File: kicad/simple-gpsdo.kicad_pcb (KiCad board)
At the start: 2 copper layers, 119.5 x 74.5 mm, 103 parts, among them J1 PPS_OUT, J2 PWR, J3 ISP, J4 GPS_NEO, J5 GPS_IN, J6 10MHz_OUT, J7 NEO-6M, J8 10MHz_OUT, J9 USB_C, Q1 DMP3099L, SW1 RST, U1 BD50FC0FP-E2, U2 ATmega32U4-AU, U3 MC74HC390, U4 CD74HC4046AM96, U5 BD50FC0FP-E2, U6 LM7171, U7 LM7171, U8 LM35-D, U9 AP62301WU-7, Y1 16MHz, Y2 NV47X

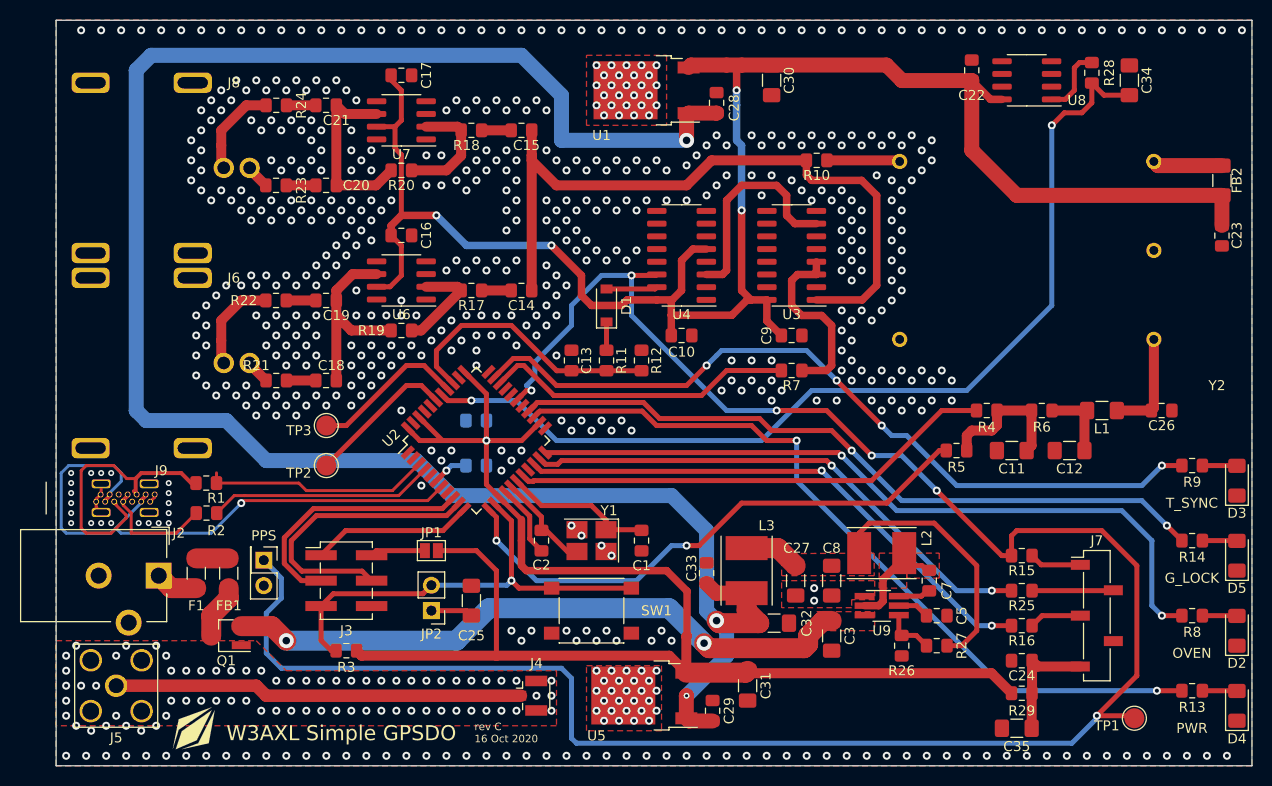
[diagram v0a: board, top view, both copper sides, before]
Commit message: schematic cleanup and re-plot of gerber files
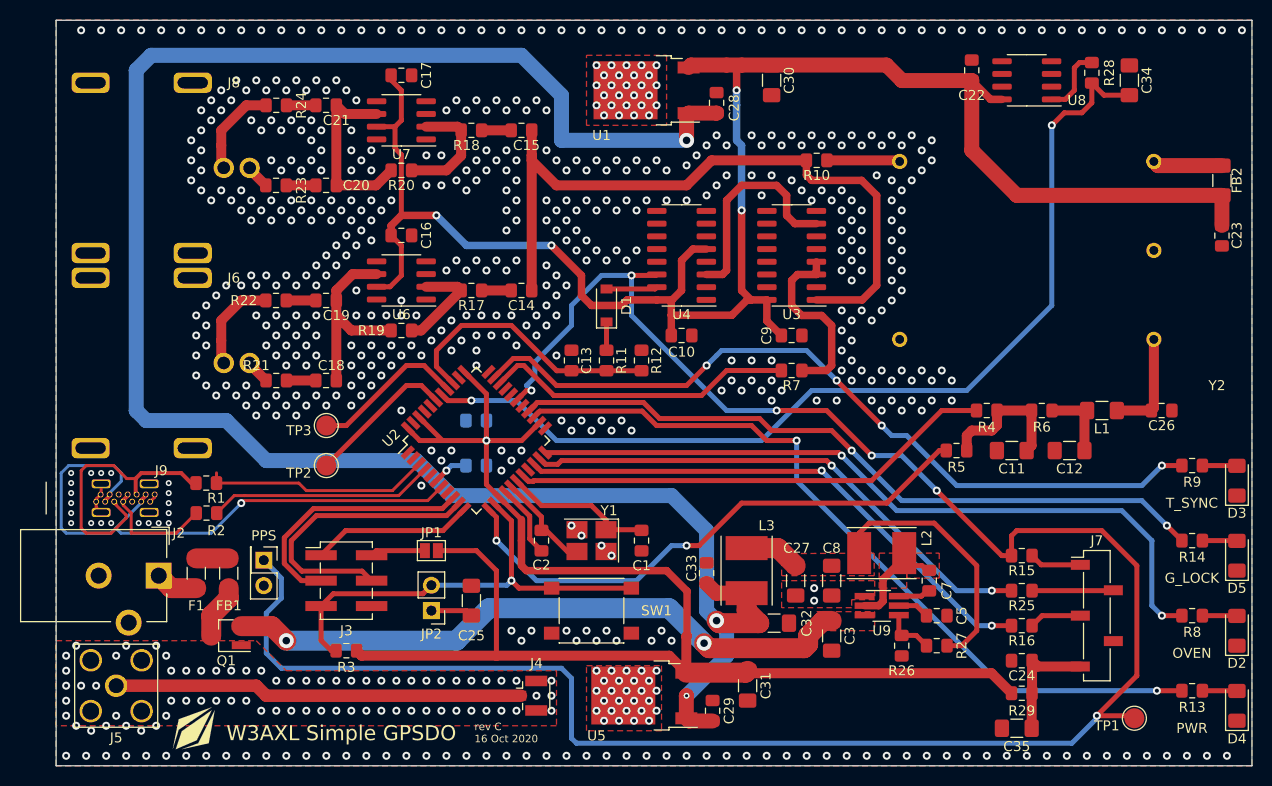
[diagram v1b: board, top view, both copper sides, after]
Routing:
- net Net-(J9-PadA7): track 28.6 -> 28.1 mm
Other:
- rule via_min_size: 0.45 -> 0.6
